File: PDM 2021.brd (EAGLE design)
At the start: 82.5 x 101.6 mm, 28 parts

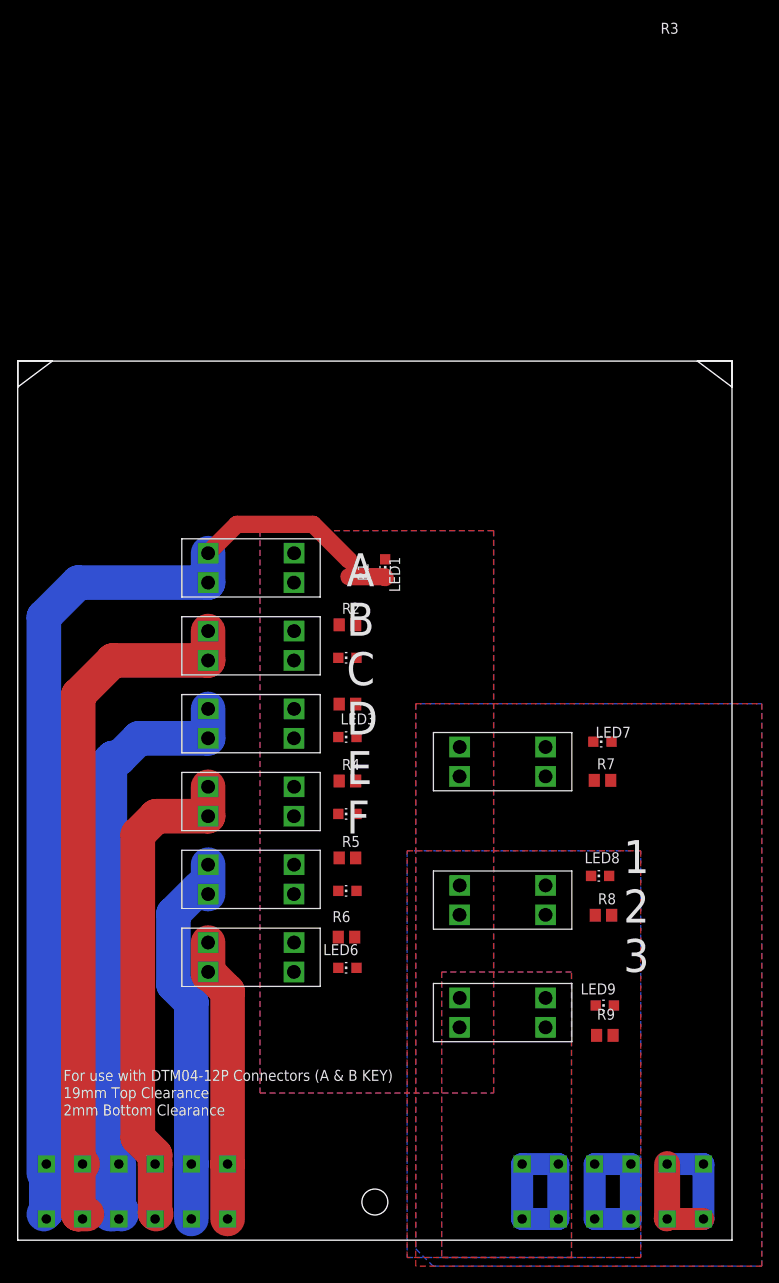
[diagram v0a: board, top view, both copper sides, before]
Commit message: Add files via upload
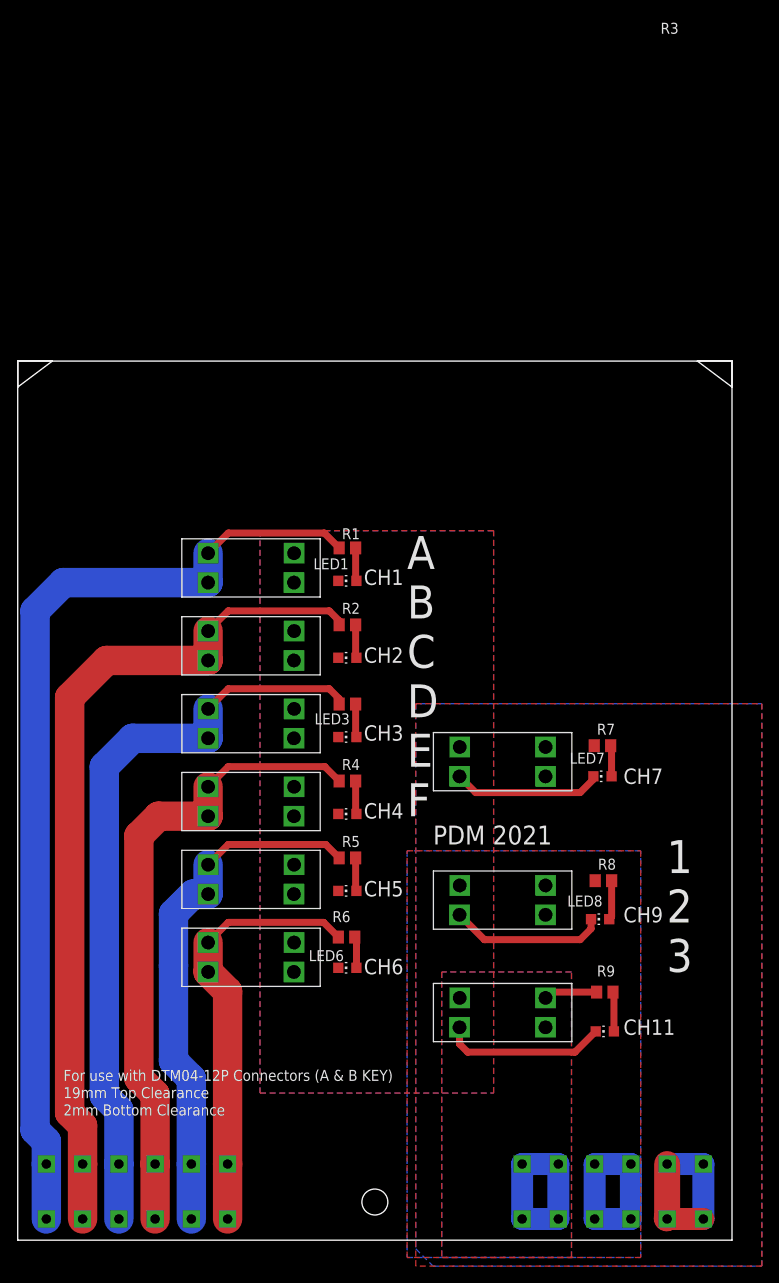
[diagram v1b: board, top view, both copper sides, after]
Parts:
- moved LED8 5.00 mm to (67.3, 38.4)
- moved R9 5.00 mm to (67.8, 29.9)
- moved LED1 4.60 mm to (38.1, 77.5), turned to 90 degrees
- moved LED7 4.00 mm to (67.6, 54.9)
- moved R7 4.00 mm to (67.6, 58.4)
- moved R8 4.00 mm to (67.7, 42.8)
- moved LED9 3.00 mm to (67.8, 25.4)
- moved R1 2.39 mm to (38.1, 81.3), turned to 0 degrees
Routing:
- net COMMON: track 0.00 -> 54.3 mm
- net CH5: track 43.8 -> 61.2 mm
- net CH6: track 32.8 -> 49.6 mm
- net CH4: track 57.7 -> 74.2 mm
- net CH2: track 82.7 -> 99.1 mm
- net CH3: track 75.1 -> 86.9 mm
- net CH11: track 21.1 -> 27.3 mm
- net N$1: track 0.00 -> 4.58 mm
- net N$2: track 0.00 -> 4.57 mm
- net N$6: track 0.00 -> 3.85 mm
- net N$5: track 0.00 -> 3.85 mm
- net N$8: track 0.00 -> 3.85 mm
- net N$7: track 0.00 -> 3.85 mm
- net N$4: track 0.00 -> 3.63 mm
- net N$3: track 0.00 -> 3.58 mm
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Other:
- board text added: "CH1"
- board text added: "CH11"
- board text added: "CH2"
- board text added: "CH3"
- board text added: "CH4"
- board text added: "CH5"
- board text added: "CH6"
- board text added: "CH7"
- board text added: "CH9"
- board text added: "PDM 2021"
